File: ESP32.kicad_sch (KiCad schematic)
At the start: 12 parts, among them J1 USB_C_4-LAYER_PADS, U1 ESP32-C6-WROOM-1-NARROW, U4 ESP32-C6FH4

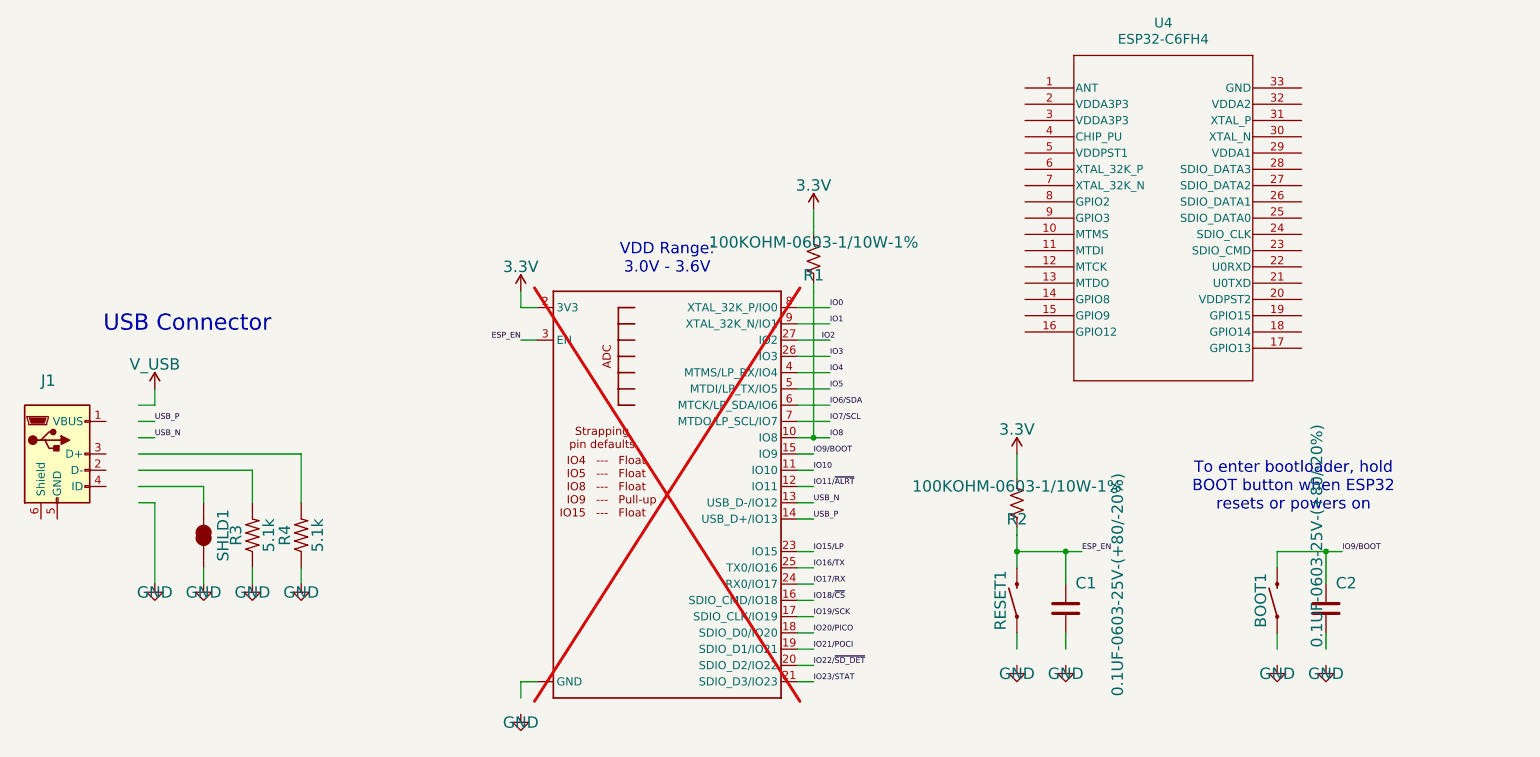
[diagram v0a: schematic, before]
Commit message: Modify ESP32
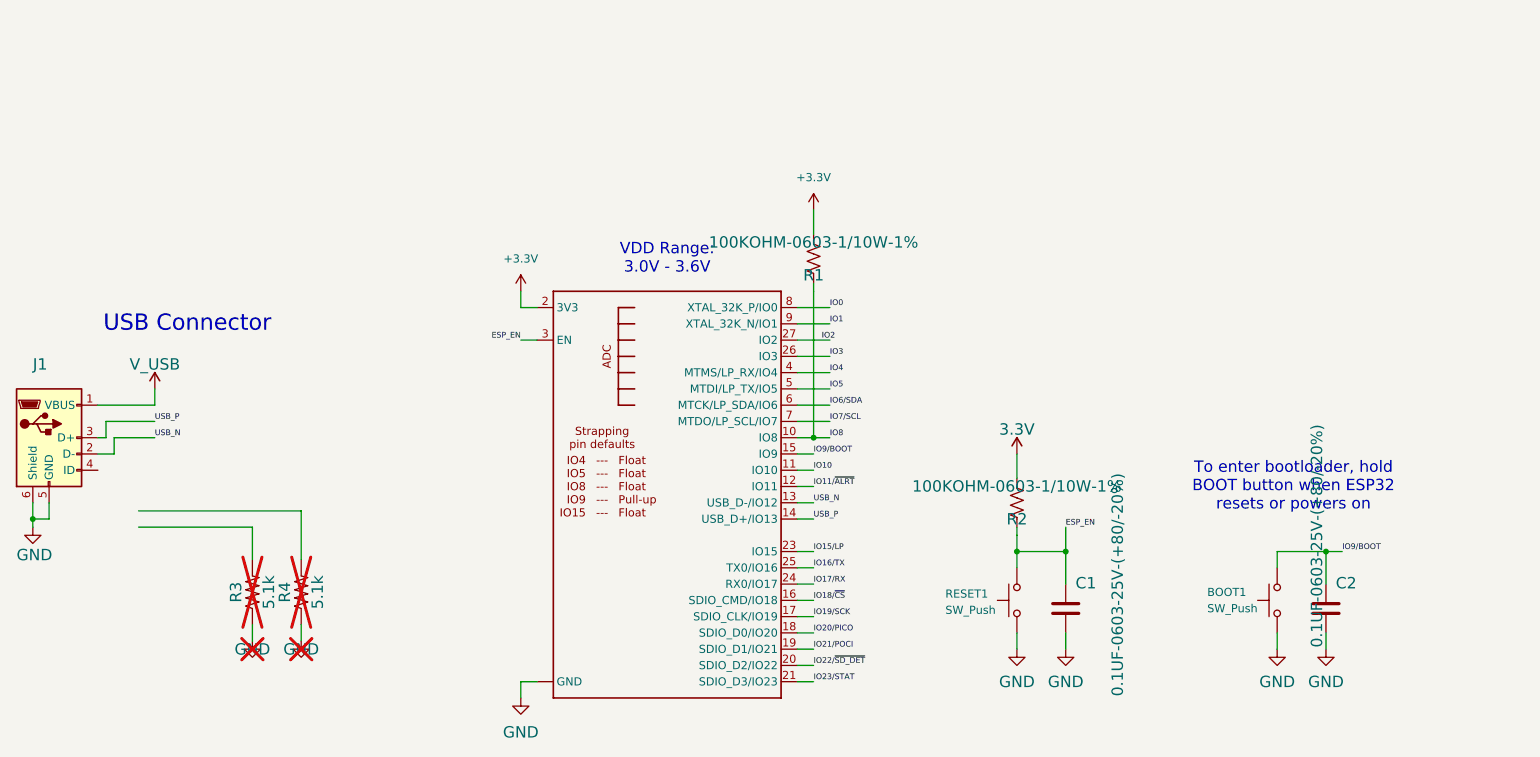
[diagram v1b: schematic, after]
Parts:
- removed BOOT1, RESET1: MOMENTARY-SWITCH-SPST-SMD-4.6X2.8MM, Button_Switch_SMD:SW_Push_1P1T_XKB_TS-1187A, symbol Thing_Plus_ESP32_C6-eagle-import:MOMENTARY-SWITCH-SPST-SMD-4.6X2.8MM
- removed SHLD1: JUMPER-SMT_2_NC_TRACE_SILK, Thing_Plus_ESP32_C6:SMT-JUMPER_2_NC_TRACE_SILK, symbol Thing_Plus_ESP32_C6-eagle-import:JUMPER-SMT_2_NC_TRACE_SILK
- removed U4: ESP32-C6FH4, uSlime-libs:QFN32_ESP32_EXP, symbol uSlime:ESP32-C6FH4
- added BOOT1, RESET1: SW_Push, Button_Switch_SMD:SW_SPST_B3U-1000P-B, symbol uSlime:SW_Push
- J1: footprint Thing_Plus_ESP32_C6:USB-C-16P_4LAYER-PADS -> Connector_USB:USB_Micro-B_Amphenol_10103594-0001LF_Horizontal
- R3, R4: now not fitted
- U1: footprint Thing_Plus_ESP32_C6:ESP32-C6-WROOM-1-NARROW -> PCM_Espressif:ESP32-C6-MINI-1; now fitted
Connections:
- net 3.3V: no longer R1.2, U1.2 (3V3)
- net ESP_EN: now also RESET1.2
- net GND: now also C1.2, C2.2, J1.5 (GND), J1.6 (Shield), U1.1 (GND), U1.28 (GND), U1.29 (GND), U1.30 (GND), U1.31 (GND), U1.32 (GND), U1.33 (GND), U1.34 (GND), U1.35 (GND), U1.36 (GND), U1.37 (GND), BOOT1.1, RESET1.1
- net USB_N: now also J1.2 (D-)
- net USB_P: now also J1.3 (D+)
- net V_USB: now also J1.1 (VBUS)
- net IO9/BOOT renamed IO9/BOOT
- net IO9/BOOT: now also BOOT1.2
- new net +3.3V: R1.2, U1.2 (3V3)
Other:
- moved on the sheet: J1

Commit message: update power
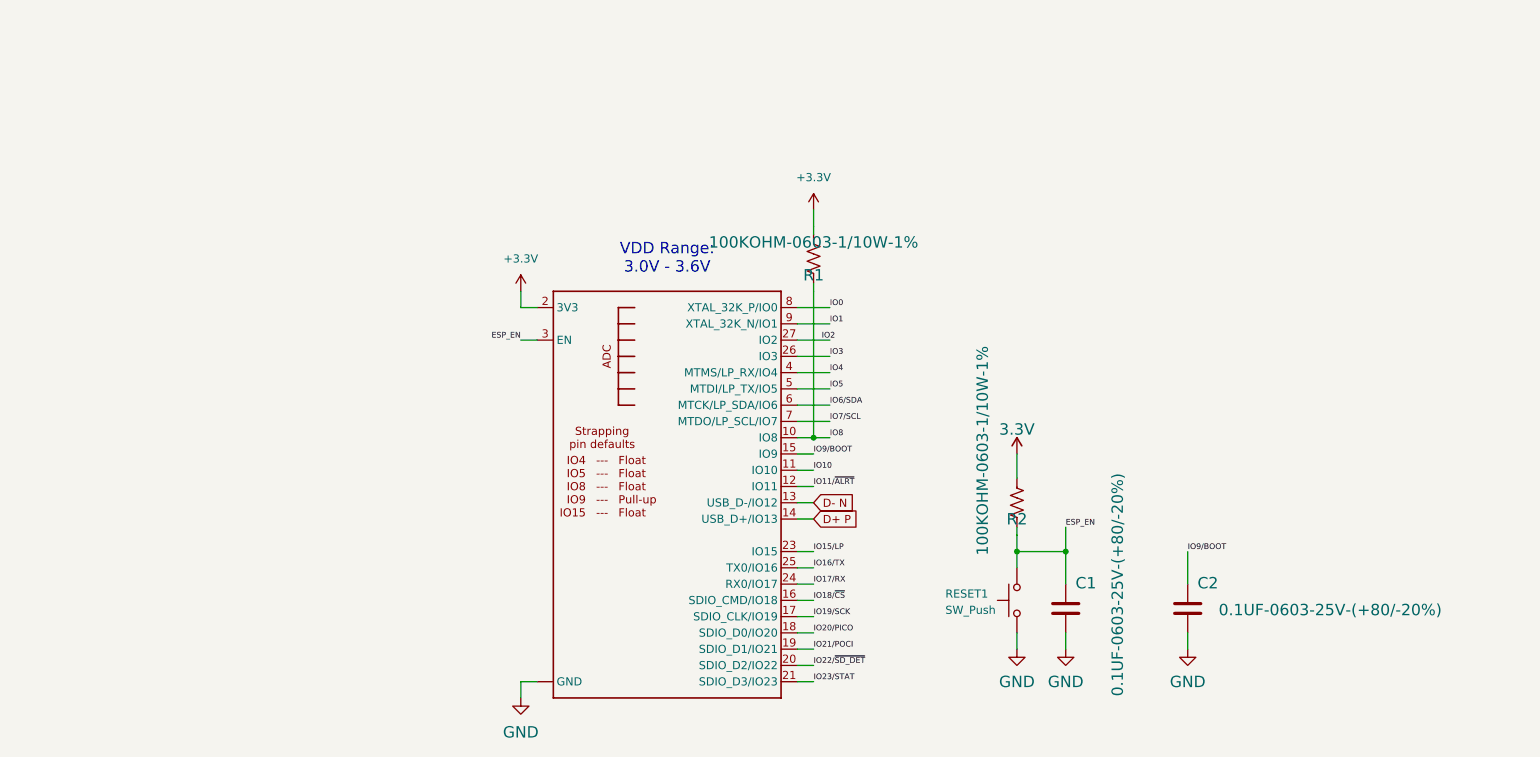
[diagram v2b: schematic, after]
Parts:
- removed BOOT1: SW_Push, Button_Switch_SMD:SW_SPST_B3U-1000P-B, symbol uSlime:SW_Push
- removed J1: USB_C_4-LAYER_PADS, Connector_USB:USB_Micro-B_Amphenol_10103594-0001LF_Horizontal, symbol Connector:USB_B_Micro
- removed R3, R4: 5.1k, Resistor_SMD:R_0603_1608Metric, symbol Thing_Plus_ESP32_C6-eagle-import:5.1KOHM5.1KOHM-0603-1/10W-1%
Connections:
- net USB_N renamed D- N
- net USB_P renamed D+ P
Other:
- note removed: "To enter bootloader, hold BOOT button when ESP32 resets or powers on"
- note removed: "USB Connector"
- moved on the sheet: C2
